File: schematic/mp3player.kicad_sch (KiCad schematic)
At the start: 38 parts, among them J1 USB_C_Receptacle_USB2.0_16P, J2 AudioJack3, J3 Conn_01x14_Socket, J4 Conn_01x02, J5 Micro_SD_Card_Det1, SW1 SW_SPDT, SW2 SW_Push, SW3 SW_Push, SW4 SW_Push, SW5 SW_Push, U1 ESP32-S3-WROOM-2, U2 PCM5102A, U3 USBLC6-2SC6, U4 TP4056-42-ESOP8, U6 AP7361C-33E

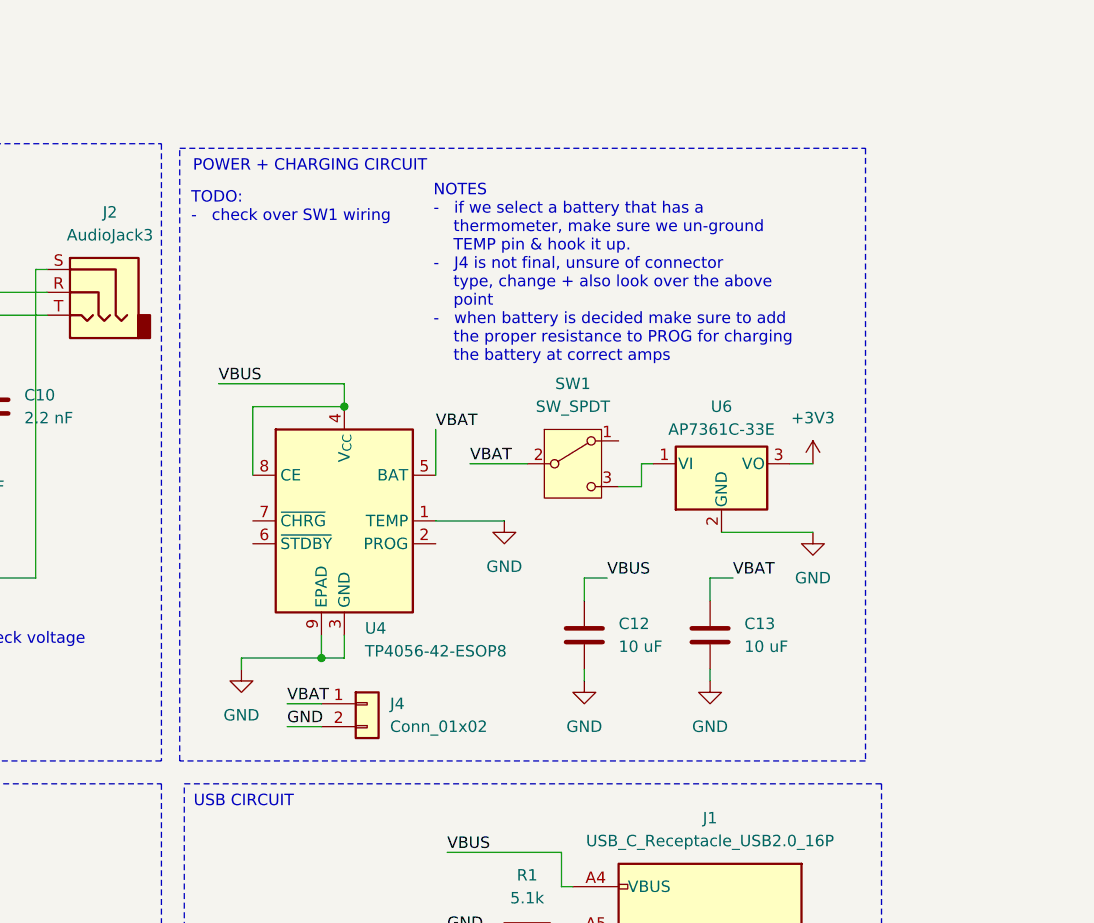
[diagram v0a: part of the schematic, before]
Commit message: added power path circuit + small cleanup
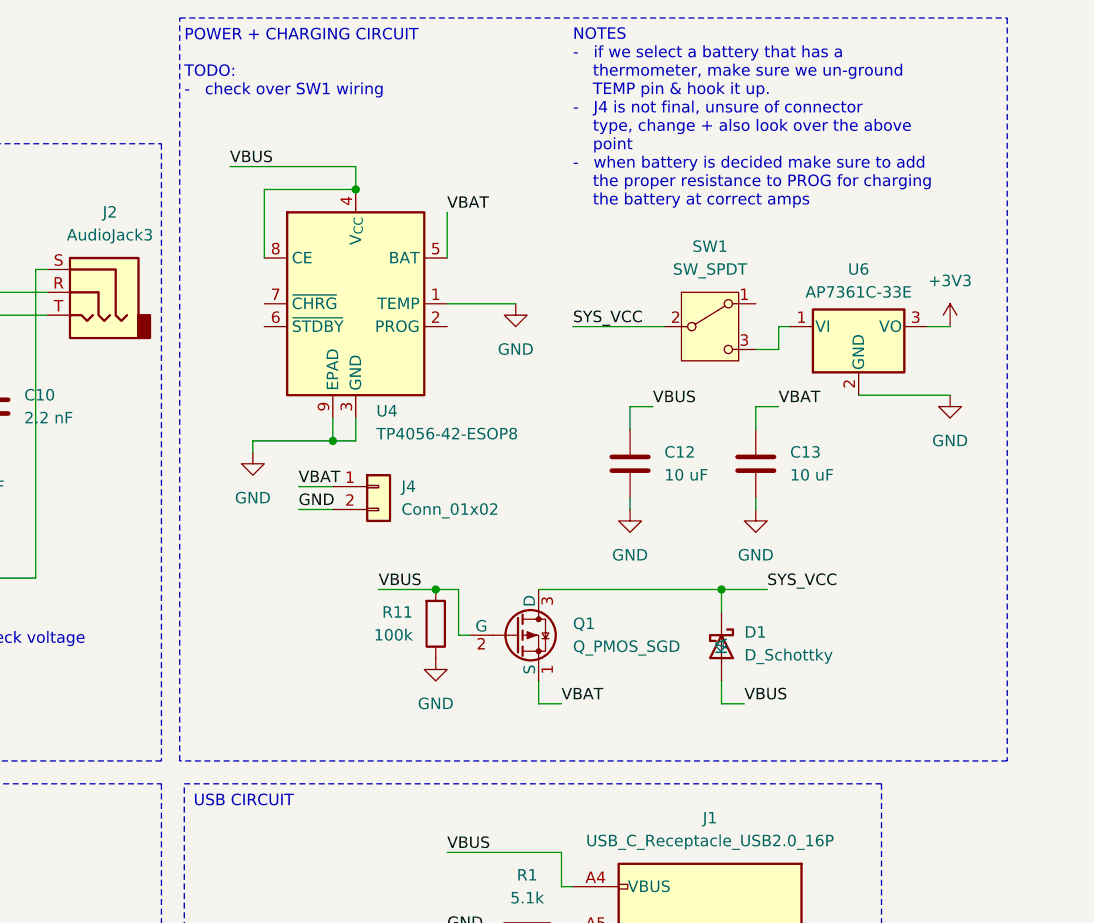
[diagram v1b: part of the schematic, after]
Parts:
- added D1: D_Schottky, Diode_SMD:D_0201_0603Metric, symbol Device:D_Schottky
- added Q1: Q_PMOS_SGD, Package_QFP:TQFP-44_10x10mm_P0.8mm, symbol Transistor_FET:Q_PMOS_SGD
- added R11: 100k, Resistor_SMD:R_0603_1608Metric, symbol Device:R
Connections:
- net GND: now also R11.1
- net VBAT: now also Q1.1 (S); no longer SW1.2 (B)
- net VBUS: now also D1.2 (A), Q1.2 (G), R11.2
- new net SYS_VCC: D1.1 (K), Q1.3 (D), SW1.2 (B)
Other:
- moved on the sheet: C12, C13, J4, SW1, U4, U6
